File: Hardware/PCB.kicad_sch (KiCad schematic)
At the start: 9 parts, among them J1 Conn_01x04_Pin, U1 ME54BS01_V1.0, U2 MCP1700x-330xxTO

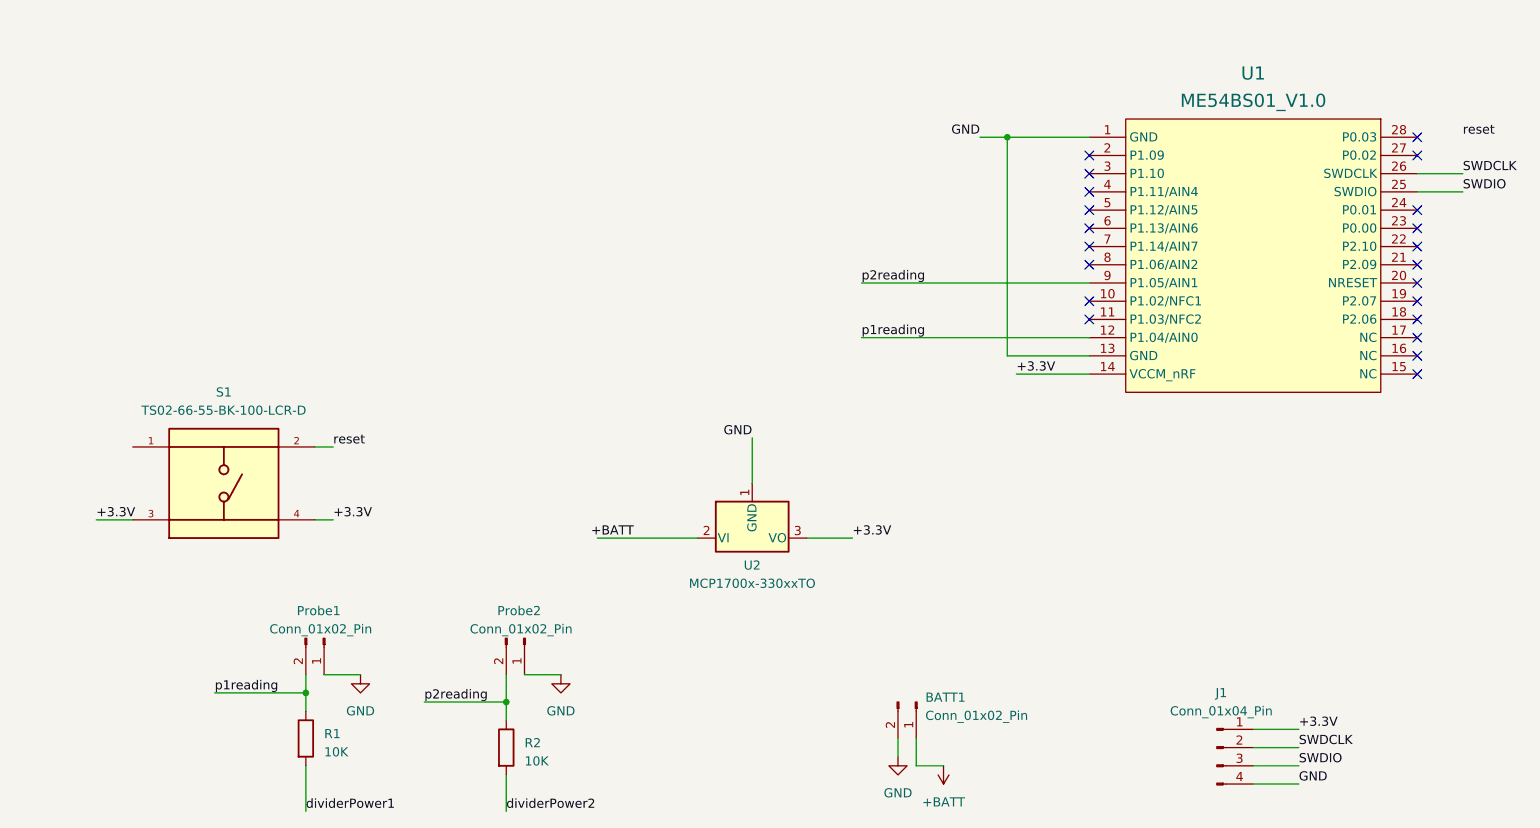
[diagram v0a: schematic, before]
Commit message: Work on PCB
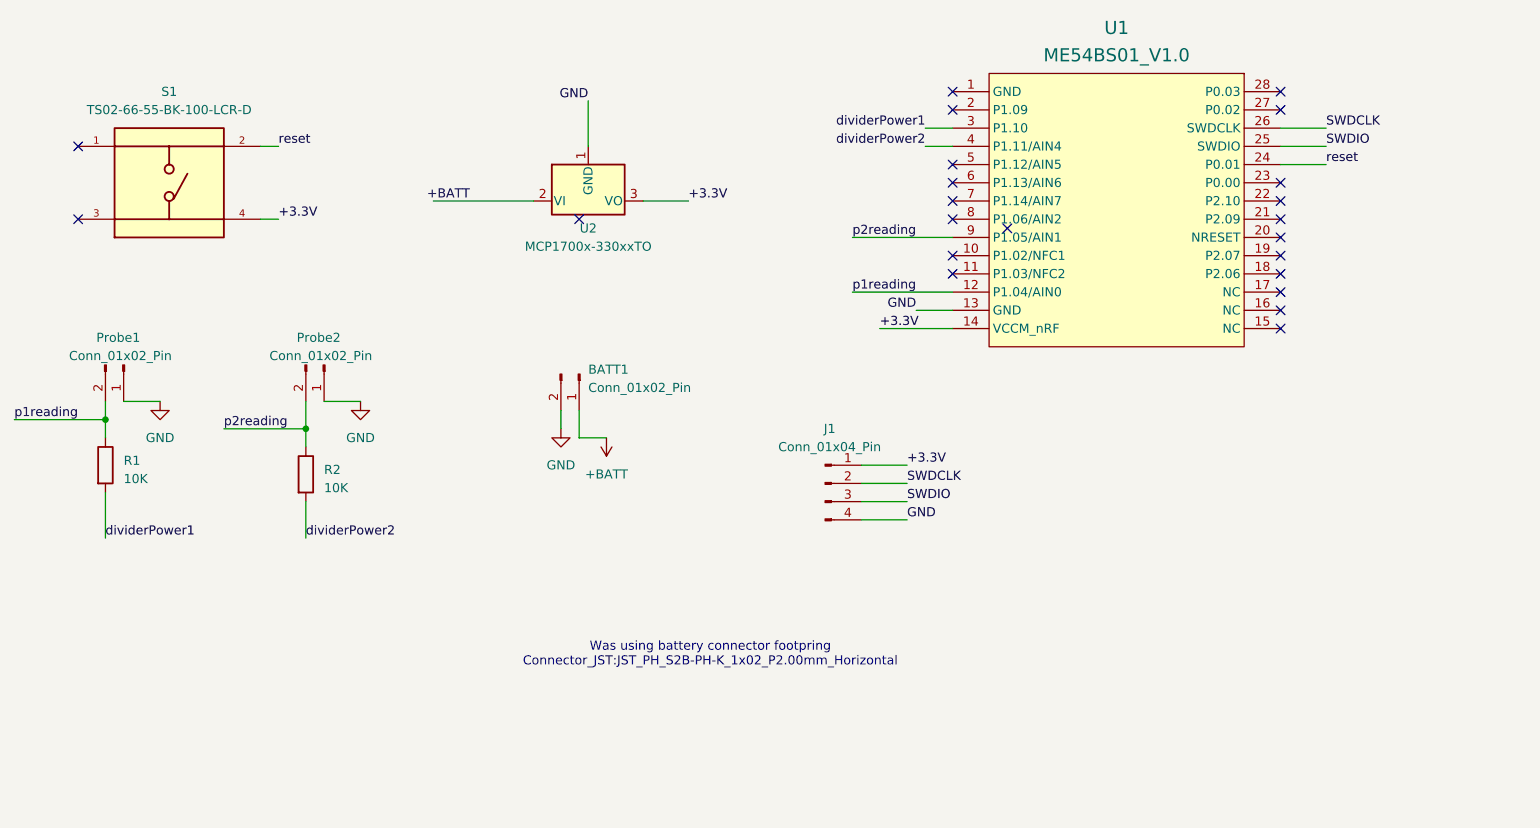
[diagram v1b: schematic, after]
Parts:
- J1: footprint (none) -> Connector_PinHeader_2.54mm:PinHeader_1x04_P2.54mm_Vertical
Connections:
- net +3.3V: no longer S1.3
- net GND: no longer U1.1 (GND)
- net dividerPower1: now also U1.3 (P1.10)
- net dividerPower2: now also U1.4 (P1.11/AIN4)
- net reset: now also U1.24 (P0.01)
- no-connect marks 21 -> 23
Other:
- note added: "Was using battery connector footpring Connector_JST:JST_PH_S2B-PH-K_1x02_P2.00mm_Horizontal"
- moved on the sheet: BATT1, J1, Probe1, Probe2, R1, R2, S1, U1, U2
